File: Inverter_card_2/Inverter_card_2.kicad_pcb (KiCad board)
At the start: 4 copper layers, 75 parts, among them J11 CONN_02X06, P0 CONN_01X03, P1 CONN_01X04, P2 CONN_01X03, P20 CONN_01X02, P3 CONN_01X03, P4 CONN_01X03, P5 CONN_01X03, P6 CONN_01X03, P7 CONN_01X03, T1 SKiiP_13ACM12V18, U11 ACS758xCB-PFF, U12 ACS758xCB-PFF, U13 ACS758xCB-PFF, U30 ISE0505A-H, U40 ACPL-C87B, U50 ACPL-C87B

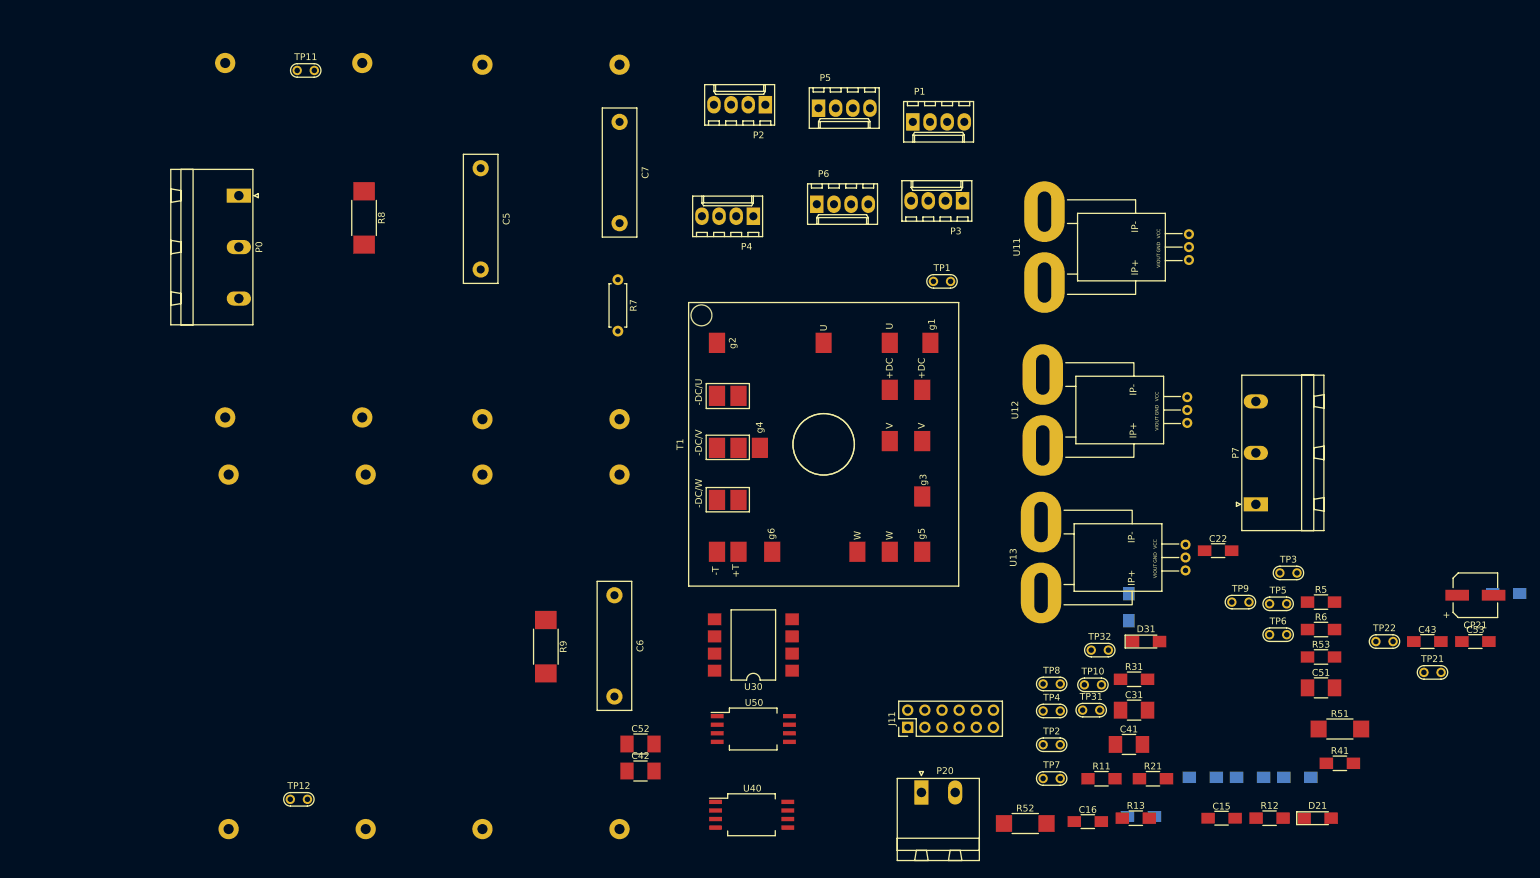
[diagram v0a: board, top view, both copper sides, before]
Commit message: A lot of work on InverterCard 2.0 pcb layout
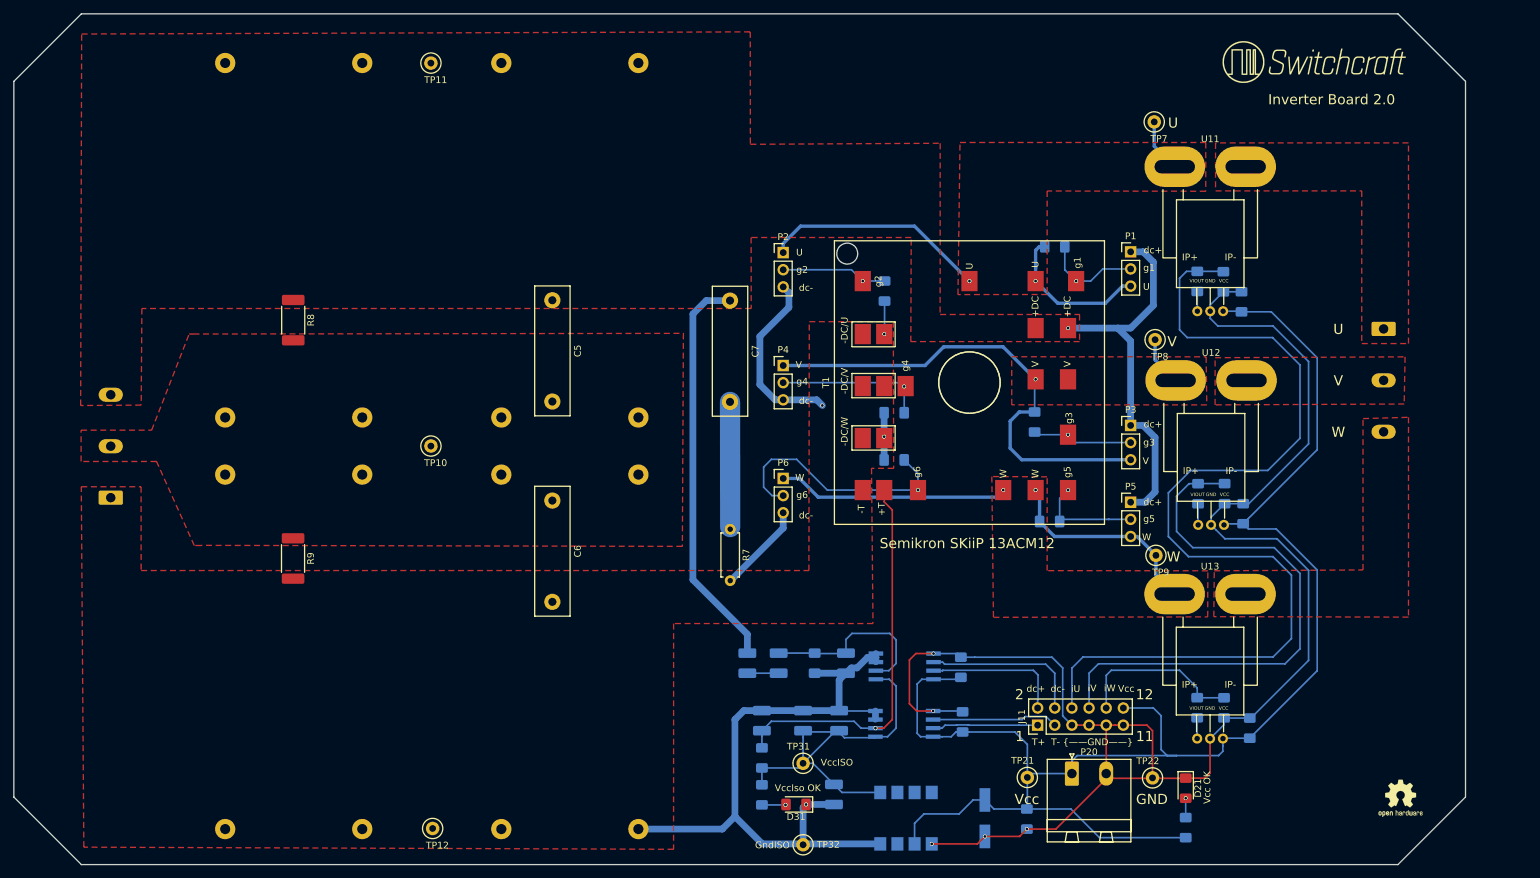
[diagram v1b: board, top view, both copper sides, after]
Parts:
- removed TP1, TP2, TP3, TP4, TP5, TP6: TEST, Measurement_Points:Test_Point
- added G***: LOGO, Switchcraft:Switchcraft_logo_10px_stroke_2000dpi, F.Cu at (227.8, 23.1)
- added REF***: OSHW-Logo2_7.3x6mm_SilkScreen, OpenSourceHardWare:OSHW-Logo2_7.3x6mm_SilkScreen, F.Cu at (240.4, 132.2)
- C11, C12, C13, C14: footprint Capacitors_SMD:C_1206_HandSoldering -> Capacitor_SMD:C_1206_3216Metric_Pad1.42x1.75mm_HandSolder
- C15, C16, C22, C43, C53: footprint Capacitors_SMD:C_1206_HandSoldering -> Capacitor_SMD:C_1206_3216Metric_Pad1.42x1.75mm_HandSolder; moved to B.Cu
- C31, C41, C42, C51, C52: footprint Capacitors_SMD:C_1210_HandSoldering -> Capacitor_SMD:C_1210_3225Metric_Pad1.42x2.65mm_HandSolder; moved to B.Cu
- C5, C6, C7: footprint Capacitors_THT:C_Rect_L19.0mm_W5.0mm_P15.00mm_MKS4 -> Capacitor_THT:C_Rect_L19.0mm_W5.0mm_P15.00mm_MKS4
- CP21: moved to B.Cu
- D21, D31: footprint LEDs:LED_1206_HandSoldering -> LED_SMD:LED_1206_3216Metric_Pad1.42x1.75mm_HandSolder
- J11: footprint Pin_Headers:Pin_Header_Straight_2x06_Pitch2.54mm -> Connector_PinHeader_2.54mm:PinHeader_2x06_P2.54mm_Vertical
- P0, P7: footprint Connectors_Phoenix:PhoenixContact_GMSTBA-G_03x7.62mm_Angled -> Connector_Phoenix_GMSTB:PhoenixContact_GMSTBA_2,5_3-G-7,62_1x03_P7.62mm_Horizontal; moved to B.Cu
- P1: value CONN_01X04 -> CONN_01X03; footprint Connectors_Molex:Molex_KK-6410-04_04x2.54mm_Straight -> Connector_PinHeader_2.54mm:PinHeader_1x03_P2.54mm_Vertical
- P2, P3, P4, P5, P6: footprint Connectors_Molex:Molex_KK-6410-04_04x2.54mm_Straight -> Connector_PinHeader_2.54mm:PinHeader_1x03_P2.54mm_Vertical
- P20: footprint PhoenixContact:MSTBA_25_2p_G_508-1757242 -> Connector_Phoenix_MSTB:PhoenixContact_MSTBA_2,5_2-G-5,08_1x02_P5.08mm_Horizontal
- R1, R2, R3, R4: footprint Resistors_SMD:R_1206_HandSoldering -> Resistor_SMD:R_1206_3216Metric_Pad1.42x1.75mm_HandSolder
- R11, R12, R13, R21, R31, R41, R5, R53, R6: footprint Resistors_SMD:R_1206_HandSoldering -> Resistor_SMD:R_1206_3216Metric_Pad1.42x1.75mm_HandSolder; moved to B.Cu
- R51, R52: footprint Resistors_SMD:R_2010_HandSoldering -> Resistor_SMD:R_1210_3225Metric_Pad1.42x2.65mm_HandSolder; moved to B.Cu
- R7: footprint Resistors_THT:R_Axial_DIN0207_L6.3mm_D2.5mm_P7.62mm_Horizontal -> Resistor_THT:R_Axial_DIN0207_L6.3mm_D2.5mm_P7.62mm_Horizontal
- R8, R9: footprint Resistors_SMD:R_2512_HandSoldering -> Resistor_SMD:R_2512_6332Metric_Pad1.52x3.35mm_HandSolder
- TP10: value TEST -> DC_MID; footprint Measurement_Points:Test_Point -> TestPoint:TestPoint_Loop_D2.50mm_Drill1.0mm_LowProfile
- TP11: value TEST -> DC+; footprint Measurement_Points:Test_Point -> TestPoint:TestPoint_Loop_D2.50mm_Drill1.0mm_LowProfile
- TP12: value TEST -> DC-; footprint Measurement_Points:Test_Point -> TestPoint:TestPoint_Loop_D2.50mm_Drill1.0mm_LowProfile
- TP21: value TEST -> VCC; footprint Measurement_Points:Test_Point -> TestPoint:TestPoint_Loop_D2.50mm_Drill1.0mm_LowProfile
- TP22: value TEST -> GND; footprint Measurement_Points:Test_Point -> TestPoint:TestPoint_Loop_D2.50mm_Drill1.0mm_LowProfile
- TP31: value TEST -> VCC_ISO; footprint Measurement_Points:Test_Point -> TestPoint:TestPoint_Loop_D2.50mm_Drill1.0mm_LowProfile
- TP32: value TEST -> GND_ISO; footprint Measurement_Points:Test_Point -> TestPoint:TestPoint_Loop_D2.50mm_Drill1.0mm_LowProfile
- TP7, TP8, TP9: footprint Measurement_Points:Test_Point -> TestPoint:TestPoint_Loop_D2.50mm_Drill1.0mm_LowProfile
- U30: footprint Housings_DIP:DIP-8_W11.48mm_SMD -> Package_DIP:SMDIP-8_W7.62mm; moved to B.Cu
- U40, U50: footprint Housings_SOIC:SSO-8_6.8x5.9mm_Pitch1.27mm_Clearance8mm -> Package_SO:SSO-8_6.8x5.9mm_P1.27mm_Clearance7mm; moved to B.Cu
- moved TP10 103.0 mm to (96.8, 80.0)
- moved TP7 98.6 mm to (203.9, 32.0)
- moved R51 88.3 mm to (143.6, 112.2), turned to 270 degrees
- moved R2 86.1 mm to (164.0, 57.1), turned to 270 degrees
- moved R41 85.6 mm to (145.8, 126.2), turned to 270 degrees
- moved R1 83.7 mm to (189.2, 50.5)
- moved C16 82.4 mm to (214.1, 55.7), turned to 270 degrees
- moved R4 80.5 mm to (165.4, 75.1)
- moved CP21 79.8 mm to (178.8, 135.1), turned to 270 degrees
- moved C53 76.3 mm to (175.3, 112.8), turned to 90 degrees
- moved R11 75.0 mm to (210.3, 55.6), turned to 270 degrees
- moved R53 75.0 mm to (153.6, 112.2), turned to 270 degrees
- moved P5 74.4 mm to (200.4, 88.3)
- moved C51 70.5 mm to (158.2, 112.2), turned to 270 degrees
- moved C43 69.9 mm to (175.5, 120.9), turned to 270 degrees
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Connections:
- J11 pad 1: VCC -> T+
- J11 pad 10: T- -> Net-(C14-Pad1)
- J11 pad 12: GND -> VCC
- J11 pad 2: GND -> Net-(J11-Pad2)
- J11 pad 3: Net-(C16-Pad1) -> T-
- J11 pad 5: Net-(C15-Pad1) -> GND
- J11 pad 6: Net-(J11-Pad6) -> Net-(C16-Pad1)
- J11 pad 7: Net-(C14-Pad1) -> GND
- J11 pad 8: T+ -> Net-(C15-Pad1)
- U30 pad 8: (no net) -> Net-(U30-Pad8)
- U50 pad 7: Net-(J11-Pad6) -> Net-(J11-Pad2)
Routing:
- net GND: track 0.00 -> 233.3 mm, vias 0 -> 6
- net VCC: track 0.00 -> 231.2 mm
- net GND_ISO: track 0.00 -> 155.5 mm, vias 0 -> 4
- net Net-(C16-Pad1): track 0.00 -> 145.0 mm
- net DC+: track 0.00 -> 116.0 mm, vias 0 -> 1
- net Net-(C15-Pad1): track 0.00 -> 83.0 mm
- net V: track 0.00 -> 79.5 mm, vias 0 -> 1
- net W: track 0.00 -> 65.4 mm, vias 0 -> 2
- net U: track 0.00 -> 63.9 mm, vias 0 -> 2
- net VCC_ISO: track 0.00 -> 59.3 mm
- net Net-(C41-Pad1): track 0.00 -> 57.9 mm, vias 0 -> 1
- net T6_g: track 0.00 -> 36.9 mm, vias 0 -> 1
- net Net-(C51-Pad1): track 0.00 -> 26.8 mm
- net Net-(C14-Pad1): track 0.00 -> 25.1 mm
- net Net-(J11-Pad4): track 0.00 -> 23.8 mm
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- added copper zone on F.Cu, net DC+
- added copper zone on F.Cu, net GND_ISO
- added copper zone on F.Cu, net Net-(C1-Pad2)
- added copper zone on F.Cu, net Net-(P7-Pad1)
- added copper zone on F.Cu, net Net-(P7-Pad2)
- added copper zone on F.Cu, net Net-(P7-Pad3)
- added copper zone on F.Cu, net U
- added copper zone on F.Cu, net V
- added copper zone on F.Cu, net W
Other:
- board outline added: 215 x 126 mm
- net class DC+: trace_width 3 -> 1
- net class UVW: trace_width 4 -> 0.5
- board text added: "1"
- board text added: "11"
- board text added: "12"
- board text added: "2"
- board text added: "DC-Link Voltage Measurement"
- board text added: "GND"
- board text added: "GndISO"
- board text added: "Inverter Board 2.0"
- board text added: "Semikron SKiiP 13ACM12"
- board text added: "T+"
- board text added: "T-"
- board text added: "U"
- board text added: "V"
- board text added: "Vcc"
- board text added: "Vcc OK"
- board text added: "VccISO"
- board text added: "VccIso OK"
- board text added: "W"
- board text added: "dc+"
- board text added: "dc-"
- board text added: "g1"
- board text added: "g2"
- board text added: "g3"
- board text added: "g4"
- board text added: "g5"
- board text added: "g6"
- board text added: "iU"
- board text added: "iV"
- board text added: "iW"
- board text added: "{——GND——}"
